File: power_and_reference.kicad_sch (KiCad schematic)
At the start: 22 parts, among them Q1 ZXTN4004KQTC, U1 BQ79616PAPRQ1

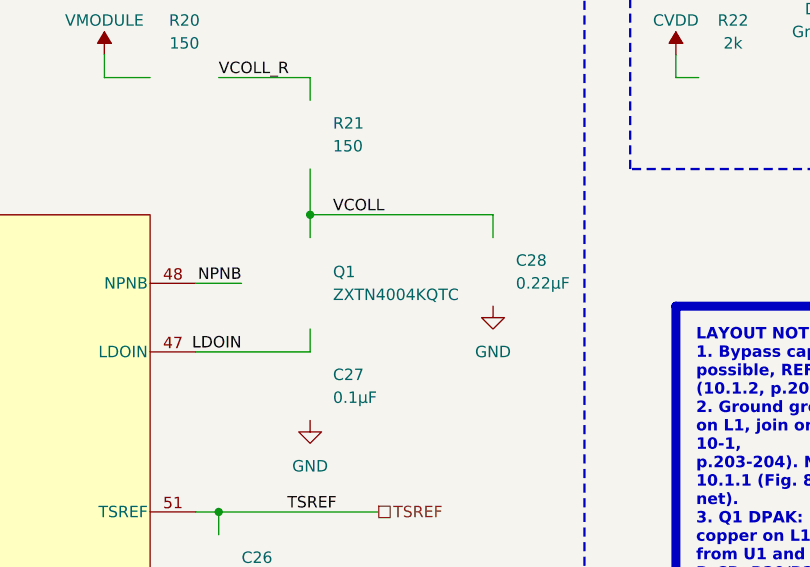
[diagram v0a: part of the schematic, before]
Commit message: SCH[Cleaning]:Updated Connectors not sure still, added sprate bat and ground connections, updated commincation conncetors. PCB[Layout]:Inital layout of compents need to fit on board size once tap connecton method is decided.
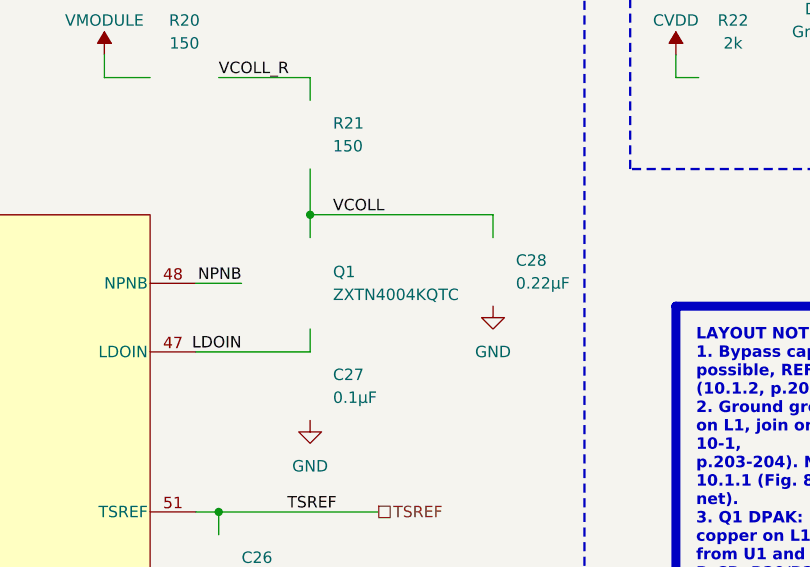
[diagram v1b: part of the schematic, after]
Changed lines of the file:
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@@
 	)
 	(symbol
-		(lib_id "remote_zxtn4004kqtc:NPN")
-		(at 167.64 78.74 0)
-		(unit 1)
-		(body_style 0)
-		(exclude_from_sim no)
-		(in_bom yes)
-		(on_board yes)
-		(in_pos_files yes)
-		(dnp no)
-		(fields_autoplaced yes)
-		(property "Reference" "Q1"
-			(at 177.8 77.4699 0)
-			(show_name no)
-			(do_not_autoplace no)
-			(effects
-				(font
-					(size 1.27 1.27)
-				)
-				(justify left)
-			)
-		)
-		(property "Value" "ZXTN4004KQTC"
-			(at 177.8 80.0099 0)
-			(show_name no)
-			(do_not_autoplace no)
-			(effects
-				(font
-					(size 1.27 1.27)
-				)
-				(justify left)
-			)
-		)
-		(property "Footprint" "remote_zxtn4004kqtc:DPAK_04KQTC_DIO"
-			(at 167.64 78.74 0)
-			(hide yes)
-			(show_name no)
-			(do_not_autoplace no)
-			(effects
-				(font
-					(size 1.27 1.27)
-				)
-			)
-		)
-		(property "Datasheet" "https://www.diodes.com/assets/Datasheets/ZXTN4004K.pdf"
-			(at 167.64 78.74 0)
-			(hide yes)
-			(show_name no)
-			(do_not_autoplace no)
-			(effects
-				(font
-					(size 1.27 1.27)
-				)
-			)
-		)
-		(property "Description" "Bipolar (BJT) Transistor NPN 150 V 1 A 3.8 W Surface Mount TO-252-3"
-			(at 167.64 78.74 0)
-			(hide yes)
-			(show_name no)
-			(do_not_autoplace no)
-			(effects
-				(font
-					(size 1.27 1.27)
-				)
-			)
-		)
-		(property "Manufacturer" "Diodes Incorporated"
-			(at 167.64 78.74 0)
-			(hide yes)
-			(show_name no)
-			(do_not_autoplace no)
-			(effects
-				(font
-					(size 1.27 1.27)
-				)
-			)
-		)
-		(property "Manufacturer Part Number" "ZXTN4004KQTC"
-			(at 167.64 78.74 0)
-			(hide yes)
-			(show_name no)
-			(do_not_autoplace no)
-			(effects
-				(font
-					(size 1.27 1.27)
-				)
-			)
-		)
-		(property "Vendor" ""
-			(at 167.64 78.74 0)
-			(hide yes)
-			(show_name no)
-			(do_not_autoplace no)
-			(effects
-				(font
-					(size 1.27 1.27)
-				)
-			)
-		)
-		(property "Vendor Part Number" ""
-			(at 167.64 78.74 0)
-			(hide yes)
-			(show_name no)
-			(do_not_autoplace no)
-			(effects
-				(font
-					(size 1.27 1.27)
-				)
-			)
-		)
-		(property "Mass (g)" ""
-			(at 167.64 78.74 0)
-			(hide yes)
-			(show_name no)
-			(do_not_autoplace no)
-			(effects
-				(font
-					(size 1.27 1.27)
-				)
-			)
-		)
-		(property "RQjC (C/W)" ""
-			(at 167.64 78.74 0)
-			(hide yes)
-			(show_name no)
-			(do_not_autoplace no)
-			(effects
-				(font
-					(size 1.27 1.27)
-				)
-			)
-		)
-		(property "RQjC_top (C/W)" ""
-			(at 167.64 78.74 0)
-			(hide yes)
-			(show_name no)
-			(do_not_autoplace no)
-			(effects
-				(font
-					(size 1.27 1.27)
-				)
-			)
-		)
-		(property "Temp_max (C)" ""
-			(at 167.64 78.74 0)
-			(hide yes)
-			(show_name no)
-			(do_not_autoplace no)
-			(effects
-				(font
-					(size 1.27 1.27)
-				)
-			)
-		)
-		(property "Temp_min (C)" ""
-			(at 167.64 78.74 0)
-			(hide yes)
-			(show_name no)
-			(do_not_autoplace no)
-			(effects
-				(font
-					(size 1.27 1.27)
-				)
-			)
-		)
-		(property "Power Dissipation (W)" ""
-			(at 167.64 78.74 0)
-			(hide yes)
-			(show_name no)
-			(do_not_autoplace no)
-			(effects
-				(font
-					(size 1.27 1.27)
-				)
-			)
-		)
-		(property "Rate" ""
-			(at 167.64 78.74 0)
-			(hide yes)
-			(show_name no)
-			(do_not_autoplace no)
-			(effects
-				(font
-					(size 1.27 1.27)
-				)
-			)
-		)
-		(property "SAP Code" ""
-			(at 167.64 78.74 0)
-			(hide yes)
-			(show_name no)
-			(do_not_autoplace no)
-			(effects
-				(font
-					(size 1.27 1.27)
-				)
-			)
-		)
-		(pin "2"
-		)
-		(pin "3"
-		)
-		(pin "1"
-		)
-		(instances
-			(project "bms_slave"
-				(path "/f9e05184-c88b-4a88-ae9c-ab2bdb32be7c/c5103ceb-5325-4a84-a025-9638a412984e/dc8544ca-af63-40ad-8cbc-696b729b5531"
-					(reference "Q1")
-					(unit 1)
-				)
-			)
-		)
-	)
-	(symbol
 		(lib_id "power:GND")
 		(at 109.22 86.36 0)
@@
 					(unit 1)
 				)
+			)
+		)
+	)
+	(symbol
+		(lib_id "remote_zxtn4004kqtc:NPN")
+		(at 167.64 78.74 0)
+		(unit 1)
+		(body_style 0)
+		(exclude_from_sim no)
+		(in_bom yes)
+		(on_board yes)
+		(in_pos_files yes)
+		(dnp no)
+		(fields_autoplaced yes)
+		(property "Reference" "Q1"
+			(at 177.8 77.47 0)
+			(show_name no)
+			(do_not_autoplace no)
+			(effects
+				(font
+					(size 1.27 1.27)
+				)
+				(justify left)
+			)
+		)
+		(property "Value" "ZXTN4004KQTC"
+			(at 177.8 80.01 0)
+			(show_name no)
+			(do_not_autoplace no)
+			(effects
+				(font
+					(size 1.27 1.27)
+				)
+				(justify left)
+			)
+		)
+		(property "Footprint" "remote_zxtn4004kqtc:DPAK_04KQTC_DIO"
+			(at 167.64 78.74 0)
+			(hide yes)
+			(show_name no)
+			(do_not_autoplace no)
+			(effects
+				(font
+					(size 1.27 1.27)
+				)
+			)
+		)
+		(property "Datasheet" "https://www.diodes.com/assets/Datasheets/ZXTN4004K.pdf"
+			(at 167.64 78.74 0)
+			(hide yes)
+			(show_name no)
+			(do_not_autoplace no)
+			(effects
+				(font
+					(size 1.27 1.27)
+				)
+			)
+		)
+		(property "Description" "Bipolar (BJT) Transistor NPN 150 V 1 A 3.8 W Surface Mount TO-252-3"
+			(at 167.64 78.74 0)
+			(hide yes)
+			(show_name no)
+			(do_not_autoplace no)
+			(effects
+				(font
+					(size 1.27 1.27)
+				)
+			)
+		)
+		(property "Manufacturer" "Diodes Incorporated"
+			(at 167.64 78.74 0)
+			(hide yes)
+			(show_name no)
+			(do_not_autoplace no)
+			(effects
+				(font
+					(size 1.27 1.27)
+				)
+			)
+		)
+		(property "Manufacturer Part Number" "ZXTN4004KQTC"
+			(at 167.64 78.74 0)
+			(hide yes)
+			(show_name no)
+			(do_not_autoplace no)
+			(effects
+				(font
+					(size 1.27 1.27)
+				)
+			)
+		)
+		(property "Vendor" ""
+			(at 167.64 78.74 0)
+			(hide yes)
+			(show_name no)
+			(do_not_autoplace no)
+			(effects
+				(font
+					(size 1.27 1.27)
+				)
+			)
+		)
+		(property "Vendor Part Number" ""
+			(at 167.64 78.74 0)
+			(hide yes)
+			(show_name no)
+			(do_not_autoplace no)
+			(effects
+				(font
+					(size 1.27 1.27)
+				)
+			)
+		)
+		(property "Mass (g)" ""
+			(at 167.64 78.74 0)
+			(hide yes)
+			(show_name no)
+			(do_not_autoplace no)
+			(effects
+				(font
+					(size 1.27 1.27)
+				)
+			)
+		)
+		(property "RQjC (C/W)" ""
+			(at 167.64 78.74 0)
+			(hide yes)
+			(show_name no)
+			(do_not_autoplace no)
+			(effects
+				(font
+					(size 1.27 1.27)
+				)
+			)
+		)
+		(property "RQjC_top (C/W)" ""
+			(at 167.64 78.74 0)
+			(hide yes)
+			(show_name no)
+			(do_not_autoplace no)
+			(effects
+				(font
+					(size 1.27 1.27)
+				)
+			)
+		)
+		(property "Temp_max (C)" ""
+			(at 167.64 78.74 0)
+			(hide yes)
+			(show_name no)
+			(do_not_autoplace no)
+			(effects
+				(font
+					(size 1.27 1.27)
+				)
+			)
+		)
+		(property "Temp_min (C)" ""
+			(at 167.64 78.74 0)
+			(hide yes)
+			(show_name no)
+			(do_not_autoplace no)
+			(effects
+				(font
+					(size 1.27 1.27)
+				)
+			)
+		)
+		(property "Power Dissipation (W)" ""
+			(at 167.64 78.74 0)
+			(hide yes)
+			(show_name no)
+			(do_not_autoplace no)
+			(effects
+				(font
+					(size 1.27 1.27)
+				)
+			)
+		)
+		(property "Rate" ""
+			(at 167.64 78.74 0)
+			(hide yes)
+			(show_name no)
+			(do_not_autoplace no)
+			(effects
+				(font
+					(size 1.27 1.27)
+				)
+			)
+		)
+		(property "SAP Code" ""
+			(at 167.64 78.74 0)
+			(hide yes)
+			(show_name no)
+			(do_not_autoplace no)
+			(effects
+				(font
+					(size 1.27 1.27)
+				)
+			)
+		)
+		(pin "2"
+		)
+		(pin "3"
+		)
+		(pin "1"
+		)
+		(instances
+			(project "bms_slave"
+				(path "/f9e05184-c88b-4a88-ae9c-ab2bdb32be7c/c5103ceb-5325-4a84-a025-9638a412984e/dc8544ca-af63-40ad-8cbc-696b729b5531"
+					(reference "Q1")
+					(unit 1)
+				)
